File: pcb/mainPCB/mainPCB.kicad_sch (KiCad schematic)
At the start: 0 parts

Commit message: wip pccb
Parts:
- added U1: ESP32-S3-DevKitC, PCM_Espressif:ESP32-S3-DevKitC, symbol PCM_Espressif:ESP32-S3-DevKitC
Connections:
- new net: U1.1 (3V3), U1.2 (3V3)
- new net: U1.22 (GND), U1.23 (GND), U1.24 (GND), U1.44 (GND)
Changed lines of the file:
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@@
 	(generator_version "9.0")
 	(paper "A4")
+	(symbol
+		(lib_id "PCM_Espressif:ESP32-S3-DevKitC")
+		(at 129.54 97.79 0)
+		(unit 1)
+		(exclude_from_sim no)
+		(in_bom yes)
+		(on_board yes)
+		(dnp no)
+		(fields_autoplaced yes)
+		(property "Reference" "U1"
+			(at 131.6833 143.51 0)
+			(effects
+				(font
+					(size 1.27 1.27)
+				)
+				(justify left)
+			)
+		)
+		(property "Value" "ESP32-S3-DevKitC"
+			(at 131.6833 146.05 0)
+			(effects
+				(font
+					(size 1.27 1.27)
+				)
+				(justify left)
+			)
+		)
+		(property "Footprint" "PCM_Espressif:ESP32-S3-DevKitC"
+			(at 129.54 154.94 0)
+			(effects
+				(font
+					(size 1.27 1.27)
+				)
+				(hide yes)
+			)
+		)
+		(property "Datasheet" ""
+			(at 69.85 100.33 0)
+			(effects
+				(font
+					(size 1.27 1.27)
+				)
+				(hide yes)
+			)
+		)
+		(property "Description" "ESP32-S3-DevKitC"
+			(at 129.54 97.79 0)
+			(effects
+				(font
+					(size 1.27 1.27)
+				)
+				(hide yes)
+			)
+		)
+		(pin "13"
+		)
+		(pin "7"
+		)
+		(pin "4"
+		)
+		(pin "31"
+		)
+		(pin "16"
+		)
+		(pin "11"
+		)
+		(pin "40"
+		)
+		(pin "20"
+		)
+		(pin "32"
+		)
+		(pin "35"
+		)
+		(pin "17"
+		)
+		(pin "39"
+		)
+		(pin "2"
+		)
+		(pin "24"
+		)
+		(pin "1"
+		)
+		(pin "6"
+		)
+		(pin "37"
+		)
+		(pin "15"
+		)
+		(pin "44"
+		)
+		(pin "19"
+		)
+		(pin "23"
+		)
+		(pin "34"
+		)
+		(pin "26"
+		)
+		(pin "22"
+		)
+		(pin "30"
+		)
+		(pin "8"
+		)
+		(pin "33"
+		)
+		(pin "43"
+		)
+		(pin "9"
+		)
+		(pin "36"
+		)
+		(pin "28"
+		)
+		(pin "12"
+		)
+		(pin "5"
+		)
+		(pin "41"
+		)
+		(pin "21"
+		)
+		(pin "38"
+		)
+		(pin "27"
+		)
+		(pin "18"
+		)
+		(pin "3"
+		)
+		(pin "14"
+		)
+		(pin "42"
+		)
+		(pin "29"
+		)
+		(pin "25"
+		)
+		(pin "10"
+		)
+		(instances
+			(project ""
+				(path "/27c374aa-4c81-4903-a17b-9cdb1b485207"
+					(reference "U1")
+					(unit 1)
+				)
+			)
+		)
+	)
 	(sheet_instances
 		(path "/"

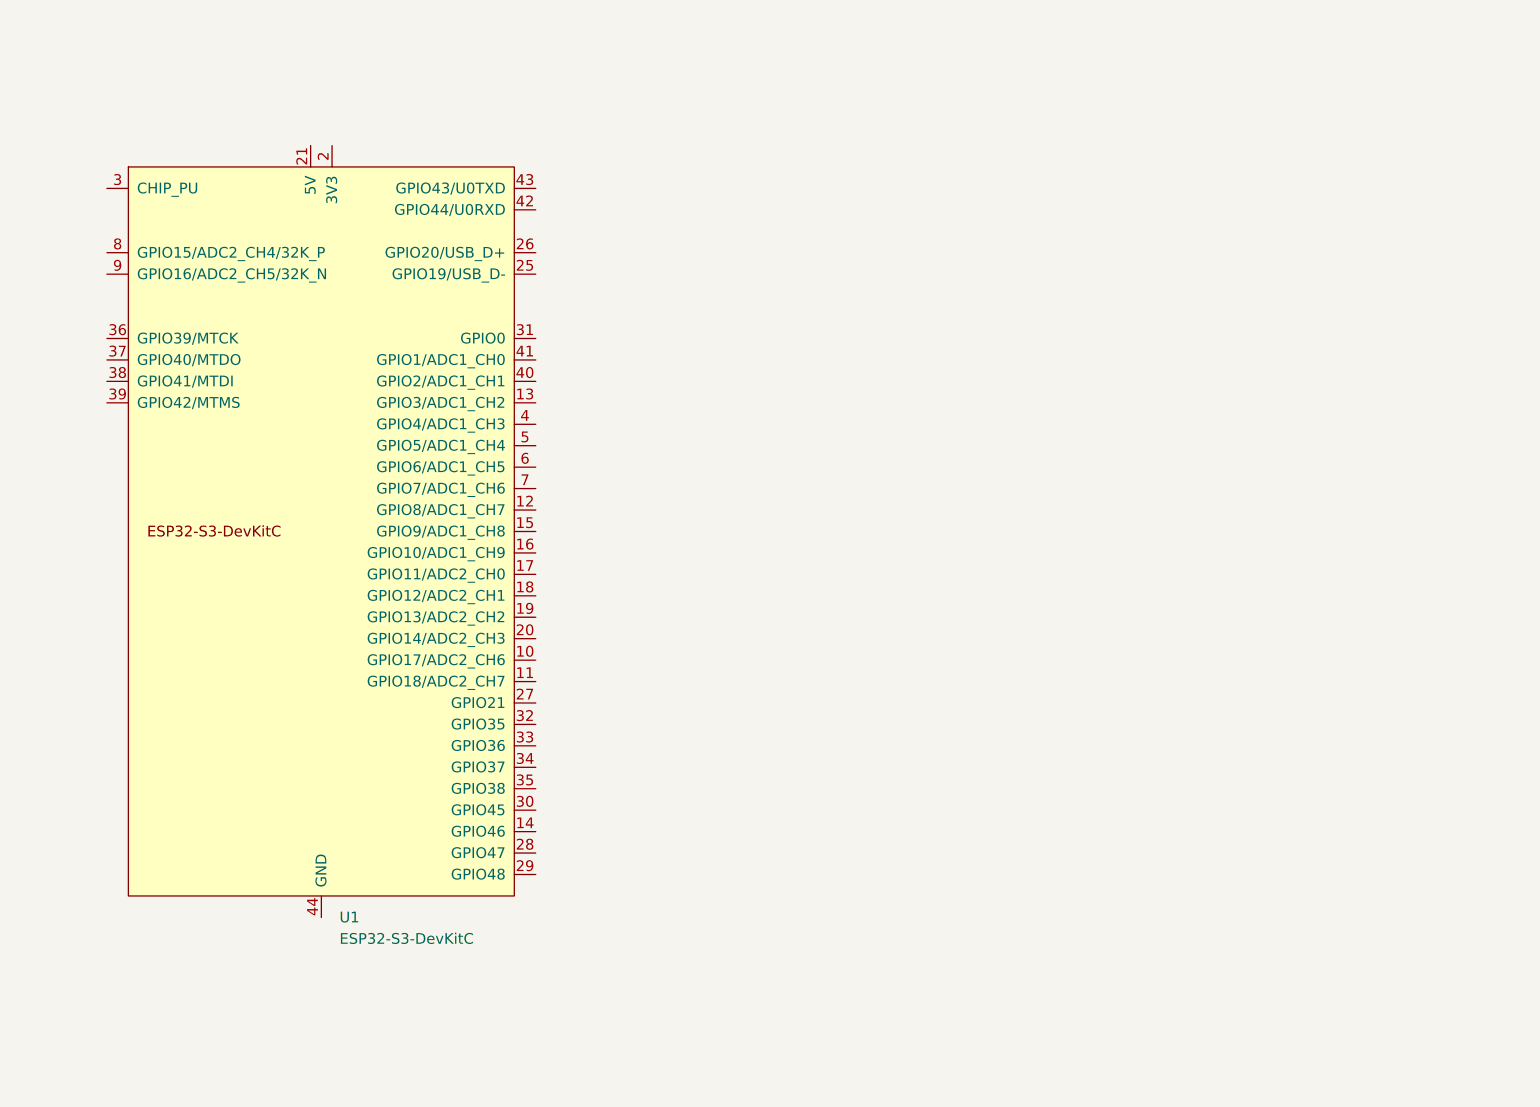
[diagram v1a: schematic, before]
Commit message: oskur, cette personne fait sûrement n'imp mais ne s'en aperçois même pas (découvrez son histoire)
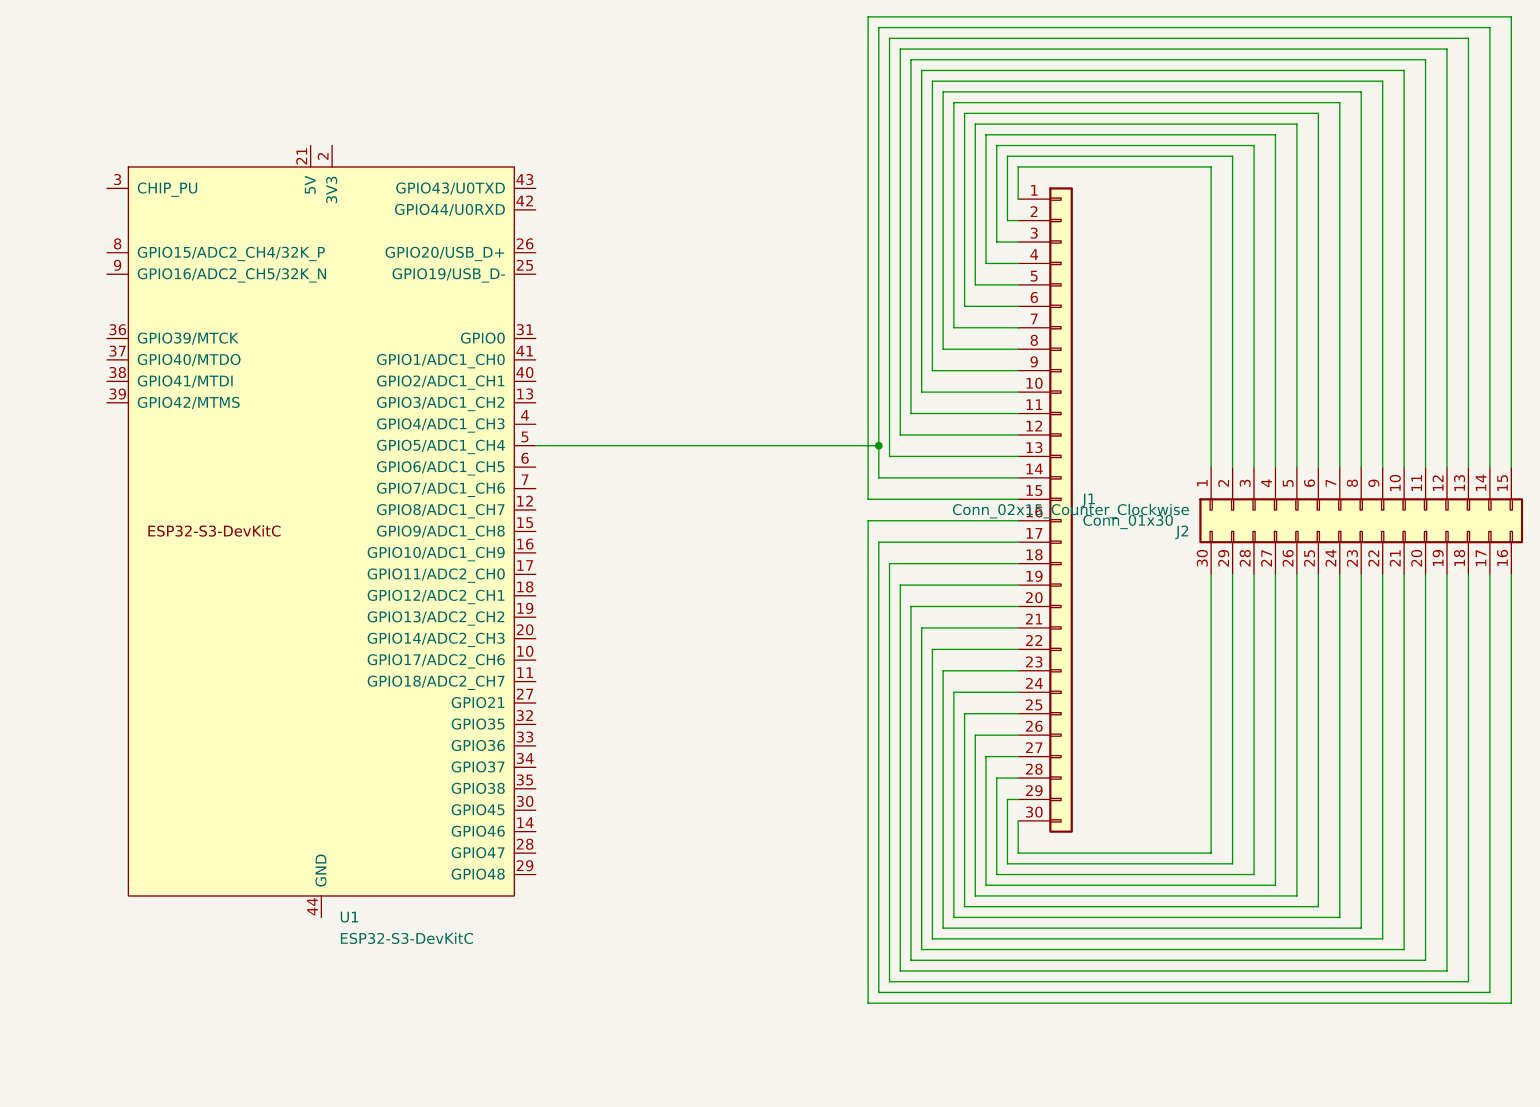
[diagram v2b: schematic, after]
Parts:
- added J1: Conn_01x30, Chris:FPC_30_Dell_0.8mm_no0, symbol Connector_Generic:Conn_01x30
- added J2: Conn_02x15_Counter_Clockwise, Connector_PinHeader_2.54mm:PinHeader_2x15_P2.54mm_Vertical, symbol Connector_Generic:Conn_02x15_Counter_Clockwise
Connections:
- net at U1.5 (GPIO5/ADC1_CH4): now also J1.14 (Pin_14), J2.14 (Pin_14)
- new net: J1.1 (Pin_1), J2.1 (Pin_1)
- new net: J1.10 (Pin_10), J2.10 (Pin_10)
- new net: J1.11 (Pin_11), J2.11 (Pin_11)
- new net: J1.12 (Pin_12), J2.12 (Pin_12)
- new net: J1.13 (Pin_13), J2.13 (Pin_13)
- new net: J1.15 (Pin_15), J2.15 (Pin_15)
- new net: J1.16 (Pin_16), J2.16 (Pin_16)
- new net: J1.17 (Pin_17), J2.17 (Pin_17)
- new net: J1.18 (Pin_18), J2.18 (Pin_18)
- new net: J1.19 (Pin_19), J2.19 (Pin_19)
- new net: J1.2 (Pin_2), J2.2 (Pin_2)
- new net: J1.20 (Pin_20), J2.20 (Pin_20)
- new net: J1.21 (Pin_21), J2.21 (Pin_21)
- new net: J1.22 (Pin_22), J2.22 (Pin_22)
- new net: J1.23 (Pin_23), J2.23 (Pin_23)
- new net: J1.24 (Pin_24), J2.24 (Pin_24)
- new net: J1.25 (Pin_25), J2.25 (Pin_25)
- new net: J1.26 (Pin_26), J2.26 (Pin_26)
- new net: J1.27 (Pin_27), J2.27 (Pin_27)
- new net: J1.28 (Pin_28), J2.28 (Pin_28)
- new net: J1.29 (Pin_29), J2.29 (Pin_29)
- new net: J1.3 (Pin_3), J2.3 (Pin_3)
- new net: J1.30 (Pin_30), J2.30 (Pin_30)
- new net: J1.4 (Pin_4), J2.4 (Pin_4)
- new net: J1.5 (Pin_5), J2.5 (Pin_5)
- new net: J1.6 (Pin_6), J2.6 (Pin_6)
- new net: J1.7 (Pin_7), J2.7 (Pin_7)
- new net: J1.8 (Pin_8), J2.8 (Pin_8)
- new net: J1.9 (Pin_9), J2.9 (Pin_9)

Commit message: pcb: hmmm yes that's better with labels
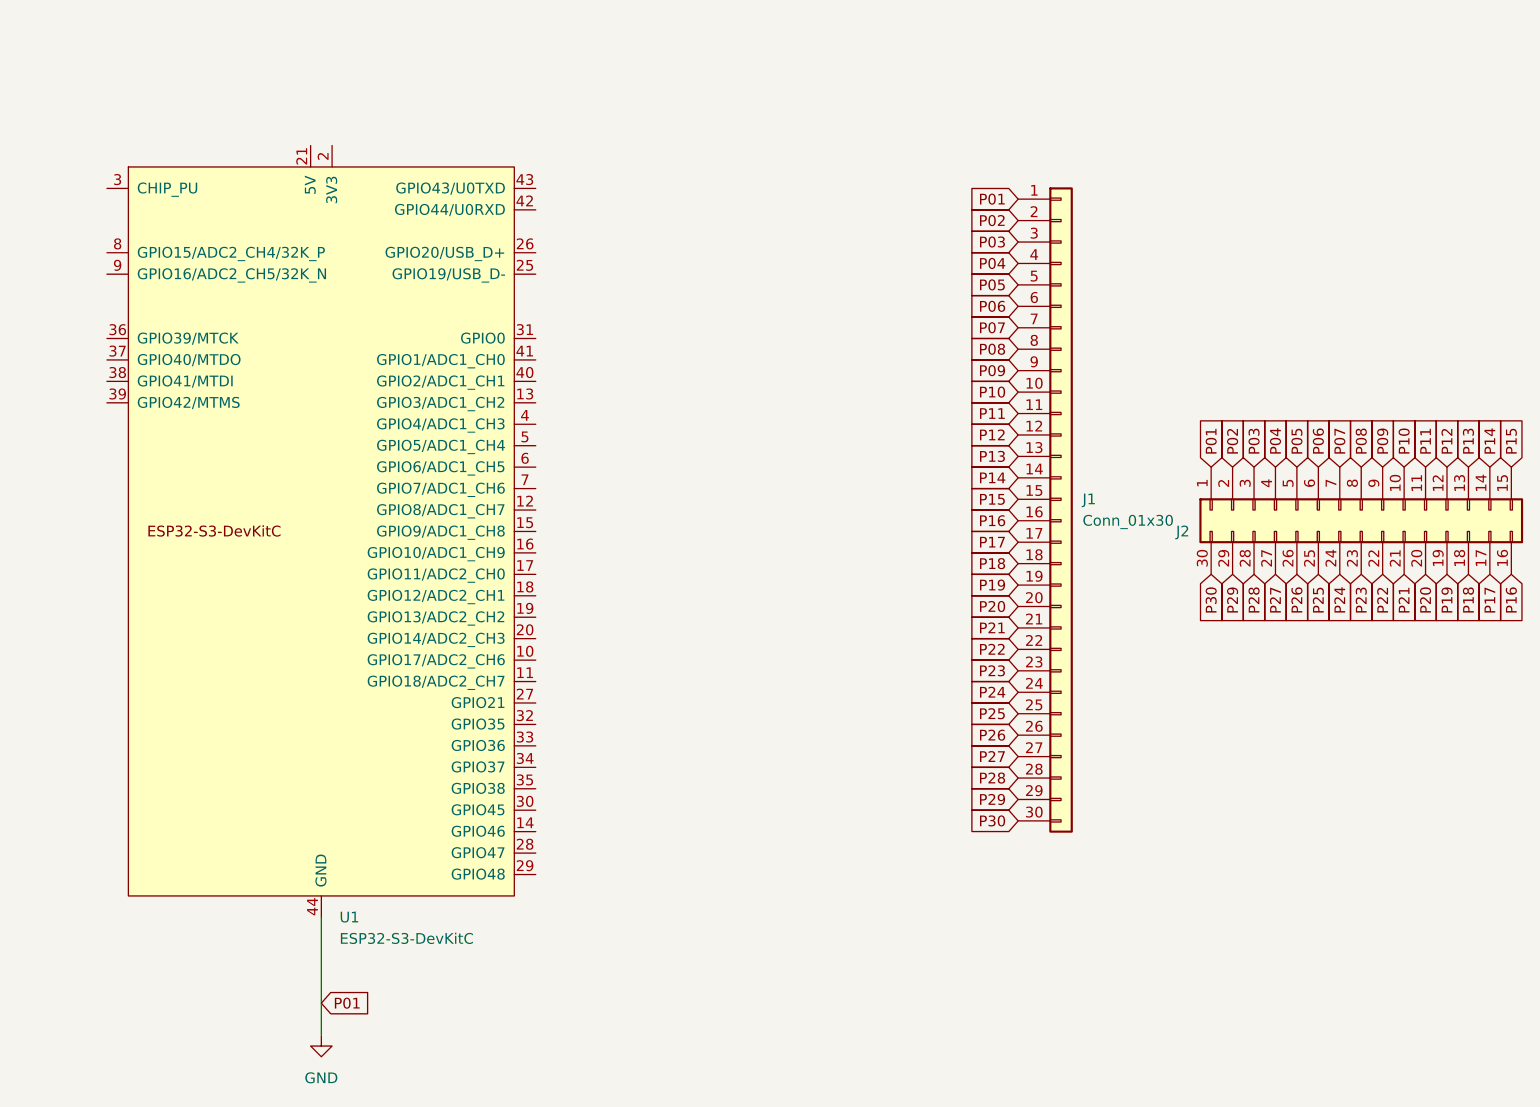
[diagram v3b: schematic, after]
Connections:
- net GND: now reaches J1.1 (Pin_1), J2.1 (Pin_1)
- net GND: now also U1.22 (GND), U1.23 (GND), U1.24 (GND), U1.44 (GND)
- net P10: now reaches J1.10 (Pin_10), J2.10 (Pin_10)
- net P11: now reaches J1.11 (Pin_11), J2.11 (Pin_11)
- net P12: now reaches J1.12 (Pin_12), J2.12 (Pin_12)
- net P13: now reaches J1.13 (Pin_13), J2.13 (Pin_13)
- net P14: now reaches J1.14 (Pin_14), J2.14 (Pin_14)
- net P14: no longer U1.5 (GPIO5/ADC1_CH4)
- net P15: now reaches J1.15 (Pin_15), J2.15 (Pin_15)
- net P16: now reaches J1.16 (Pin_16), J2.16 (Pin_16)
- net P17: now reaches J1.17 (Pin_17), J2.17 (Pin_17)
- net P18: now reaches J1.18 (Pin_18), J2.18 (Pin_18)
- net P19: now reaches J1.19 (Pin_19), J2.19 (Pin_19)
- net P02: now reaches J1.2 (Pin_2), J2.2 (Pin_2)
- net P20: now reaches J1.20 (Pin_20), J2.20 (Pin_20)
- net P21: now reaches J1.21 (Pin_21), J2.21 (Pin_21)
- net P22: now reaches J1.22 (Pin_22), J2.22 (Pin_22)
- net P23: now reaches J1.23 (Pin_23), J2.23 (Pin_23)
- net P24: now reaches J1.24 (Pin_24), J2.24 (Pin_24)
- net P25: now reaches J1.25 (Pin_25), J2.25 (Pin_25)
- net P26: now reaches J1.26 (Pin_26), J2.26 (Pin_26)
- net P27: now reaches J1.27 (Pin_27), J2.27 (Pin_27)
- net P28: now reaches J1.28 (Pin_28), J2.28 (Pin_28)
- net P29: now reaches J1.29 (Pin_29), J2.29 (Pin_29)
- net P03: now reaches J1.3 (Pin_3), J2.3 (Pin_3)
- net P30: now reaches J1.30 (Pin_30), J2.30 (Pin_30)
- net P04: now reaches J1.4 (Pin_4), J2.4 (Pin_4)
- net P05: now reaches J1.5 (Pin_5), J2.5 (Pin_5)
- net P06: now reaches J1.6 (Pin_6), J2.6 (Pin_6)
- net P07: now reaches J1.7 (Pin_7), J2.7 (Pin_7)
- net P08: now reaches J1.8 (Pin_8), J2.8 (Pin_8)
- net P09: now reaches J1.9 (Pin_9), J2.9 (Pin_9)

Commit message: wip: starting pcb wiring
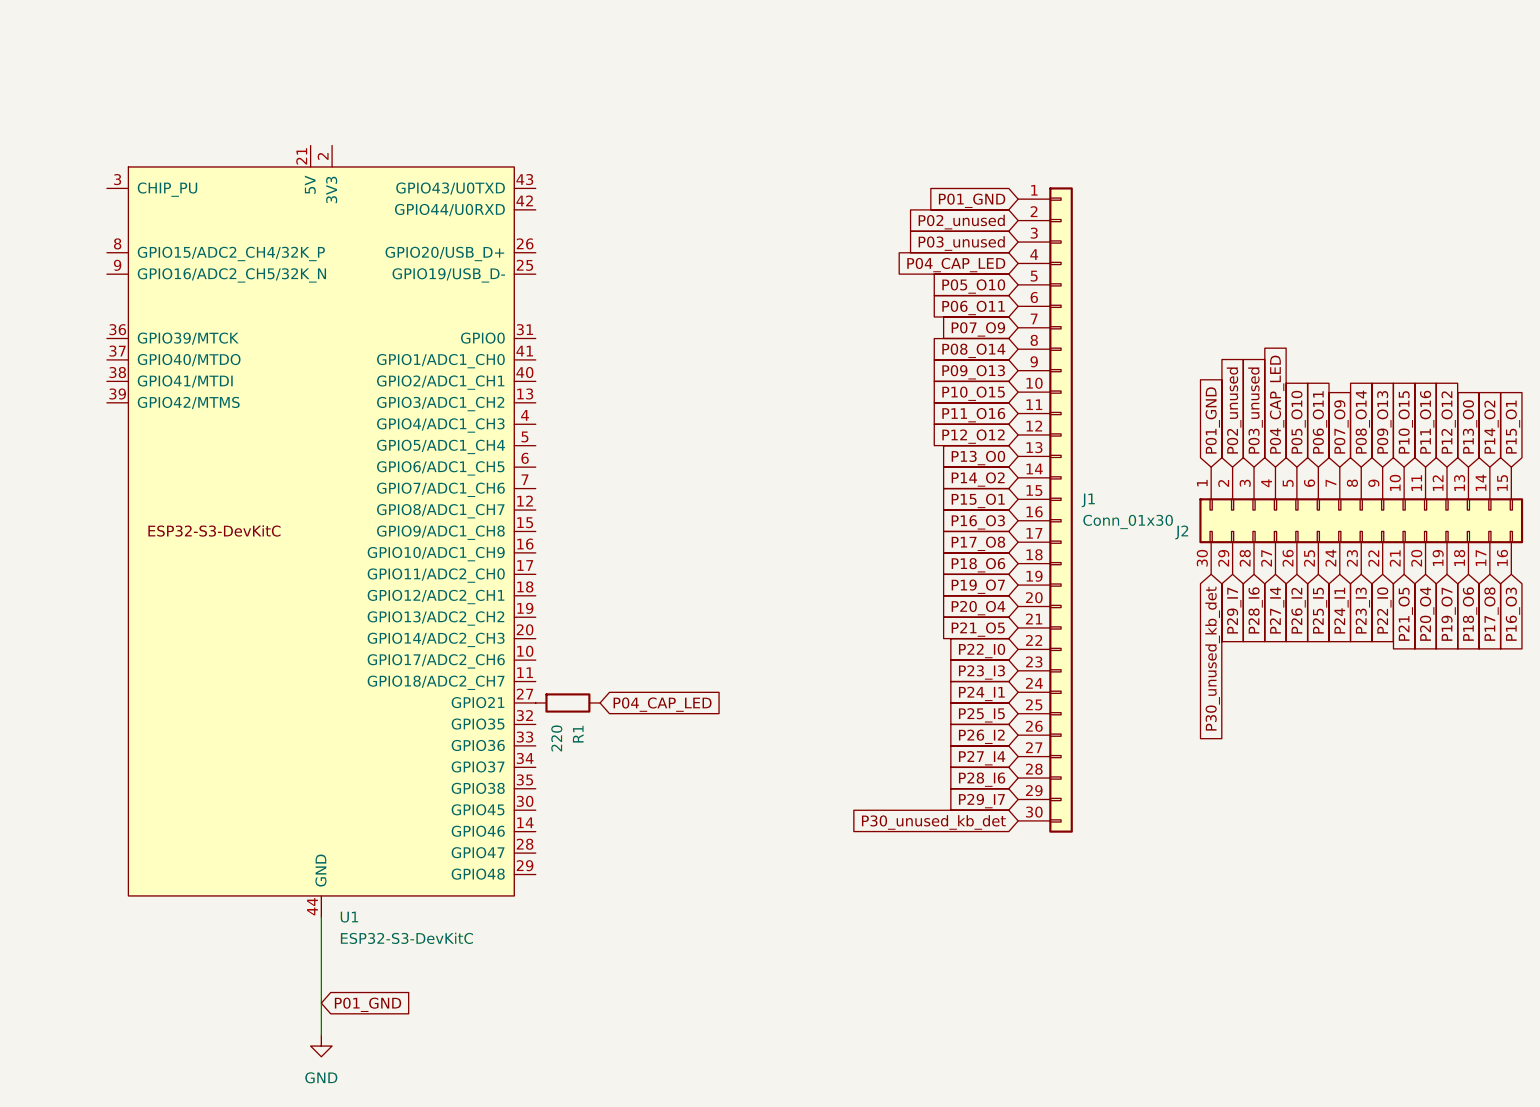
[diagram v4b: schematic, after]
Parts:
- added R1: 220, Resistor_THT:R_Axial_DIN0207_L6.3mm_D2.5mm_P10.16mm_Horizontal, symbol Device:R
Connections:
- net at U1.27 (GPIO21): now also R1.2
- net P02 renamed P02_unused
- net P03 renamed P03_unused
- net P04 renamed P04_CAP_LED
- net P04_CAP_LED: now also R1.1
- net P05 renamed P05_O10
- net P06 renamed P06_O11
- net P07 renamed P07_O9
- net P08 renamed P08_O14
- net P09 renamed P09_O13
- net P10 renamed P10_O15
- net P11 renamed P11_O16
- net P12 renamed P12_O12
- net P13 renamed P13_O0
- net P14 renamed P14_O2
- net P15 renamed P15_O1
- net P16 renamed P16_O3
- net P17 renamed P17_O8
- net P18 renamed P18_O6
- net P19 renamed P19_O7
- net P20 renamed P20_O4
- net P21 renamed P21_O5
- net P22 renamed P22_I0
- net P23 renamed P23_I3
- net P24 renamed P24_I1
- net P25 renamed P25_I5
- net P26 renamed P26_I2
- net P27 renamed P27_I4
- net P28 renamed P28_I6
- net P29 renamed P29_I7
- net P30 renamed P30_unused_kb_det
